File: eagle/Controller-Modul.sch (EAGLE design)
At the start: 53 parts, among them IC2 7805TV, Q6 BC550C, Q7 BC560, U1 ATTINY85-20S, X1 MKDSN1,5/2-5,08, X2 MKDSN1,5/2-5,08, X4 MKDSN1,5/2-5,08

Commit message: pcb design
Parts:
- removed C1, C5, C6: 100nF, rcl:C-EUC0805
- removed C2: 100µ, resistor:CPOL-EUE2.5-7
- removed C3: (no value), rcl:C-EUC0603K
- removed C4: 1000µ, rcl:CPOL-EUE3.5-8
- removed D1: 18V, diode:ZENER-DIODESOD80C
- removed D2: (no value), diode:ZENER-DIODESOT23
- removed D3: 1N4004, diode:1N4004
- removed IC1: (no value), v-reg:LM317TS
- removed IC2: 7805TV, linear:7805TV
- removed LED1: (no value), led:LED3MM
- removed Q2, Q3, Q4, Q5: (no value), transistor-power:PMOSFET_NTO220BV
- removed Q6: BC550C, transistor-npn:BC550C
- removed Q7: BC560, transistor-pnp:BC560
- removed R15: 1k, resistor:R-EU_R1206
- removed R16, R18, R19: 33k, resistor:R-EU_R1206
- removed R17: 10k, resistor:R-EU_R1206
- removed R20: 100k, rcl:R-EU_R1206
- removed R21: (no value), pot:TRIM_EU-PT10
- removed R5, R6, R7: (no value), resistor:R-EU_0207/10
- removed TR1, TR2: (no value), trafo:EI38-1
- removed U$1: GLEICHRICHTER, Gleichrichter:GLEICHRICHTER
- removed U1: ATTINY85-20S, _hhn_attiny25_45_85:ATTINY85-20S
- removed X1, X2, X4: MKDSN1,5/2-5,08, con-phoenix-508:MKDSN1,5/2-5,08
- added 1: SUMMER4, 0liver:SUMMER4
- added C10, C11: 22pF, resistor:C-EUC0603K
- added C12: 100 nF, resistor:C-EUC0603
- added C9: 1n, rcl:C-EUC0603K
- added D4, D5, D6: (no value), diode:ZENER-DIODESOT23
- added IC3: ATMEGA328P, avr-6:MEGA48/88/168-PU
- added JP10, JP4, JP6: (no value), pinhead:PINHD-1X2
- added JP5: (no value), pinhead:PINHD-1X4
- added JP7: (no value), pinhead:PINHD-1X16
- added JP8: (no value), pinhead:PINHD-2X3
- added JP9: (no value), pinhead:PINHD-1X3
- C7: value 100nF -> 1n; device rcl:C-EUC0805 -> rcl:C-EUC0603K
- C8: value 100µ -> 1n; device rcl:CPOL-EUE3.5-8 -> rcl:C-EUC0603K
- JP2: device pinhead:PINHD-2X3 -> pinhead:PINHD-1X2
- Q1: value (none) -> BC550C; device transistor-power:PMOSFET_NTO220BV -> transistor-npn:BC550C
- R10, R8: value (none) -> 300; device resistor:R-EU_0207/10 -> resistor:R-EU_R1206
- R11: value (none) -> 10k; device resistor:R-EU_0207/10 -> pot:TRIM_EU-PT10
- R12: value 100k -> 2k7; device rcl:R-EU_R1206 -> resistor:R-EU_R1206
- R13: value 10k -> 300
- R14: value 33k -> 2k7
- R2: value (none) -> 10k; device resistor:R-EU_0207/10 -> resistor:R-EU_R1206
- R3: value (none) -> 33k; device resistor:R-EU_0207/10 -> resistor:R-EU_R1206
- R4: value (none) -> 220; device resistor:R-EU_0207/10 -> resistor:R-EU_R1206
- R9: value (none) -> 2k7; device resistor:R-EU_0207/10 -> resistor:R-EU_R1206
- U$2: value GLEICHRICHTER -> ABRACON_ABM3_CRYSTALABM03_HC49; device Gleichrichter:GLEICHRICHTER -> Ava:ABRACON_ABM3_CRYSTALABM03_HC49
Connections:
- removed net +5V: C1.1, C6.1, IC2.VO, JP2.2, R12.2, U1.VCC
- removed net N$1: Q7.B, R13.2, R14.2
- removed net N$15: R15.1
- removed net N$16: Q1.D, Q2.D, Q3.D, Q4.D, Q5.D, R19.1
- removed net N$17: C4.+, C5.1, IC2.VI, U$1.+
- removed net N$19: TR1.P1, X4-1.KL
- removed net N$2: Q5.G, R11.1, R6.1
- removed net N$20: TR1.P2, X4-2.KL
- removed net N$21: TR1.S3, U$1.AC2
- removed net N$22: TR1.S4, U$1.AC1
- removed net N$23: R17.2, U1.PB3
- removed net N$25: U$2.AC2, X1-1.KL
- removed net N$29: JP1.2, R21.A
- removed net N$3: Q6.B, R16.2, R17.1
- removed net N$30: IC1.ADJ, JP1.1, R20.1
- removed net N$5: Q6.C, R13.1
- removed net N$7: Q3.G, R4.1, R9.1
- removed net N$8: C2.+, D1.C, Q7.E, R14.1, R15.2
- new net C1V: C7.2, D4.A, JP1.1, JP5.3, R8.1, R9.2
- new net C2V: C8.2, D5.A, JP5.1, R10.1, R12.2
- new net DATA0: IC3.PD2(INT0/PCINT18), JP7.11
- new net DATA1: IC3.PD3(INT1/OC2B/PCINT19), JP7.12
- new net DATA2: IC3.PD4(T0/XCK/PCINT20), JP7.13
- new net DATA3: IC3.PD5(T1/OC0B/PCINT21), JP7.14
- new net LED: IC3.PB0(ICP1/CLKO/PCINT0), R4.1
- new net N$26: IC3.PB1(OC1A/PCINT1), R1.2
- new net N$31: IC3.PD7(AIN1/PCINT23), JP9.2
- new net N$32: JP7.3, R11.S
- new net N$34: IC3.PD6(AIN0/OC0A/PCINT22), JP9.1
- new net N$47: JP7.15, R4.2
- new net RES: IC3.PC6(/RESET/PCINT14), JP8.5
- new net RS: IC3.PD0(RXD/PCINT16), JP7.4
- new net RW: IC3.PD1(TXD/PCINT17), JP7.6
- new net SENV: C9.2, D6.A, JP5.4, R13.1, R14.2
- new net VCC: C12.1, IC3.AREF, IC3.AVCC, IC3.VCC@1, JP10.2, JP7.2, JP8.2, Q1.C, R11.A
- net GND: now also 1.+, C10.2, C11.2, C12.2, IC3.AGND, IC3.GND@1, JP1.2, JP10.1, JP2.1, JP3.1, JP5.2, JP6.2, JP7.1, JP7.16, JP7.5, JP8.6, JP9.3, R11.E, R12.1, R14.1, R3.2, R9.1; no longer C1.2, C2.-, C3.2, C4.-, C5.2, C6.2, C7.2, C8.-, D1.A, D2.A, IC2.GND, JP2.6, JP3.2, LED1.C, Q6.E, R16.1, R18.1, R21.E, R21.S, U$1.-, U$2.-, U1.GND, X2-1.KL
- net MISO: now also IC3.PB4(MISO/PCINT4), JP8.1; no longer JP2.1, U1.PB1
- net MOSI: now also IC3.PB3(MOSI/OC2A/PCINT3), JP8.4; no longer JP2.4, U1.PB0
- net N$10: now also IC3.PC0(ADC0/PCINT8), JP2.2; no longer JP2.5, R12.1, U1.NRES/PB5
- net N$11: now also JP4.1, Q1.E; no longer Q1.S, Q2.S, Q3.S, Q4.S, Q5.S, R2.2, R3.2, R4.2, R5.2, R6.2
- net N$12: now also IC3.PC1(ADC1/PCINT9), JP3.2; no longer R1.2, U1.PB4
- net N$13: now also 1.-, JP4.2; no longer Q1.G, R2.1, R7.1
- net N$14: now also C7.1, D4.C, IC3.PC4(ADC4/SDA/PCINT12), R8.2; no longer C3.1, D2.C, R18.2, R19.2
- net N$18: now also C9.1, D6.C, IC3.PC2(ADC2/PCINT10), R13.2; no longer Q7.C, R10.2, R11.2, R7.2, R8.2, R9.2
- net N$24: now also C8.1, D5.C, IC3.PC3(ADC3/PCINT11), R10.2; no longer U$2.AC1, X1-2.KL
- net N$27: now also C11.1, IC3.PB7(XTAL2/TOSC2/PCINT7), U$2.2; no longer C7.1, C8.+, D3.C, IC1.IN, U$2.+
- net N$28: now also C10.1, IC3.PB6(XTAL1/TOSC1/PCINT6), U$2.1; no longer D3.A, IC1.OUT, JP3.1, R20.2, X2-2.KL
- net N$4: now also Q1.B, R2.2; no longer Q4.G, R10.1, R5.1
- net N$6: now also JP6.1; no longer LED1.A
- net N$9: now also IC3.PB2(SS/OC1B/PCINT2), R2.1; no longer Q2.G, R8.1
- net SCK: now also IC3.PB5(SCK/PCINT5), JP8.3; no longer JP2.3, U1.PB2
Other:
- note added: "5V Vcc"
- note added: "AutoSchalter"
- note added: "Con: Kondensator Supply"
- note added: "FET Treiber"
- note added: "Fußtaster"
- note added: "LED"
- note added: "SDA"
- note added: "Voltmeter"
- note added: "Volume"
- note removed: "ISP"
- moved on the sheet: C7, JP1, JP3, R1, R10, R12, R13, R14, R2, R3, R4, R8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

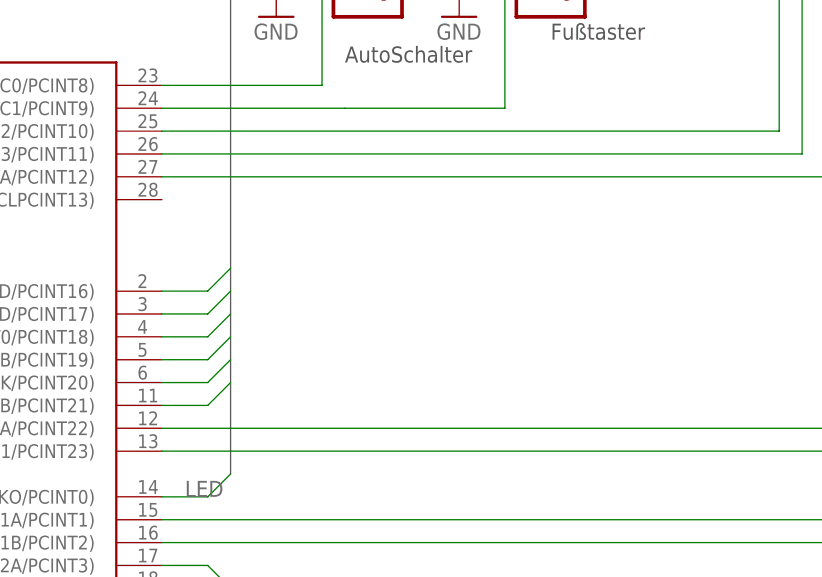
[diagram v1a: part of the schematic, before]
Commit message: Lots of schema and board changes
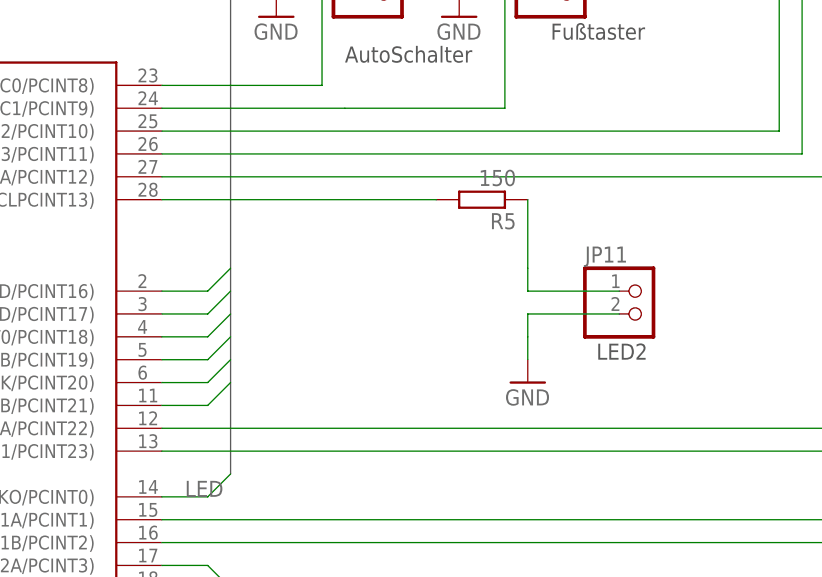
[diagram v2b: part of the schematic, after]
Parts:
- added JP11: (no value), pinhead:PINHD-1X2
- added R5: 150, rcl:R-EU_R1206
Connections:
- new net N$1: JP11.1, R5.1
- new net N$2: IC3.PC5(ADC5/SCLPCINT13), R5.2
- net GND: now also JP11.2
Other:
- note added: "LED2"
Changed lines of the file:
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@@
 <part name="JP9" library="pinhead" deviceset="PINHD-1X3" device=""/>
 <part name="GND2" library="supply1" deviceset="GND" device=""/>
+<part name="R5" library="rcl" deviceset="R-EU_" device="R1206" value="150"/>
+<part name="GND1" library="supply1" deviceset="GND" device=""/>
+<part name="JP11" library="pinhead" deviceset="PINHD-1X2" device=""/>
 </parts>
 <sheets>
@@
 <text x="144.78" y="53.34" size="1.778" layer="97">AutoSchalter</text>
 <text x="248.92" y="2.54" size="1.778" layer="97">FET Treiber</text>
+<text x="172.72" y="20.32" size="1.778" layer="97">LED2</text>
 </plain>
 <instances>
@@
 <instance part="JP9" gate="A" x="251.46" y="10.16"/>
 <instance part="GND2" gate="1" x="238.76" y="-2.54"/>
+<instance part="R5" gate="G$1" x="160.02" y="38.1" rot="R180"/>
+<instance part="GND1" gate="1" x="165.1" y="17.78"/>
+<instance part="JP11" gate="G$1" x="177.8" y="25.4"/>
 </instances>
 <busses>
@@
 <wire x1="238.76" y1="5.08" x2="238.76" y2="0" width="0.1524" layer="91"/>
 <pinref part="GND2" gate="1" pin="GND"/>
+</segment>
+<segment>
+<pinref part="GND1" gate="1" pin="GND"/>
+<wire x1="165.1" y1="22.86" x2="165.1" y2="20.32" width="0.1524" layer="91"/>
+<wire x1="165.1" y1="22.86" x2="165.1" y2="25.4" width="0.1524" layer="91"/>
+<pinref part="JP11" gate="G$1" pin="2"/>
+<wire x1="165.1" y1="25.4" x2="175.26" y2="25.4" width="0.1524" layer="91"/>
 </segment>
 </net>
@@
 </segment>
 </net>
+<net name="N$1" class="0">
+<segment>
+<pinref part="R5" gate="G$1" pin="1"/>
+<wire x1="165.1" y1="38.1" x2="165.1" y2="30.48" width="0.1524" layer="91"/>
+<pinref part="JP11" gate="G$1" pin="1"/>
+<wire x1="175.26" y1="27.94" x2="165.1" y2="27.94" width="0.1524" layer="91"/>
+<wire x1="165.1" y1="27.94" x2="165.1" y2="30.48" width="0.1524" layer="91"/>
+</segment>
+</net>
+<net name="N$2" class="0">
+<segment>
+<pinref part="R5" gate="G$1" pin="2"/>
+<pinref part="IC3" gate="1" pin="PC5(ADC5/SCLPCINT13)"/>
+<wire x1="154.94" y1="38.1" x2="124.46" y2="38.1" width="0.1524" layer="91"/>
+</segment>
+</net>
